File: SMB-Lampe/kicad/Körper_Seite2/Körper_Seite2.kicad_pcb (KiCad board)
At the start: 2 copper layers, 121.9 x 96.3 mm, 32 parts, among them J1 Conn_01x01_Pin, J2 Conn_01x01_Pin, J3 Conn_01x01_Pin

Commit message: Alle Platinen sind fertig zur Fertigung
Aus diesem Stand folgt das erste fertig leuchtende Pferd
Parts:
- C1, C2, C3, C4, C5, C6, C7, C8, C9: footprint Capacitor_SMD:C_0201_0603Metric -> Capacitor_SMD:C_0603_1608Metric_Pad1.08x0.95mm_HandSolder
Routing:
- net GND: track 351.6 -> 358.0 mm
- net Net-(D8-DOUT): track 34.9 -> 37.5 mm
- net +5V: track 207.2 -> 209.1 mm
- net Net-(D7-DOUT): track 82.5 -> 80.9 mm
- net /Data_OUT_Hinterbein_vorne_Seite1: track 71.5 -> 72.8 mm
- net (no net): track 3.40 -> 2.50 mm
- net Net-(D1-DOUT): track 45.8 -> 46.5 mm
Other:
- board size 121.9 x 96.3 mm -> 281.3 x 135.5 mm

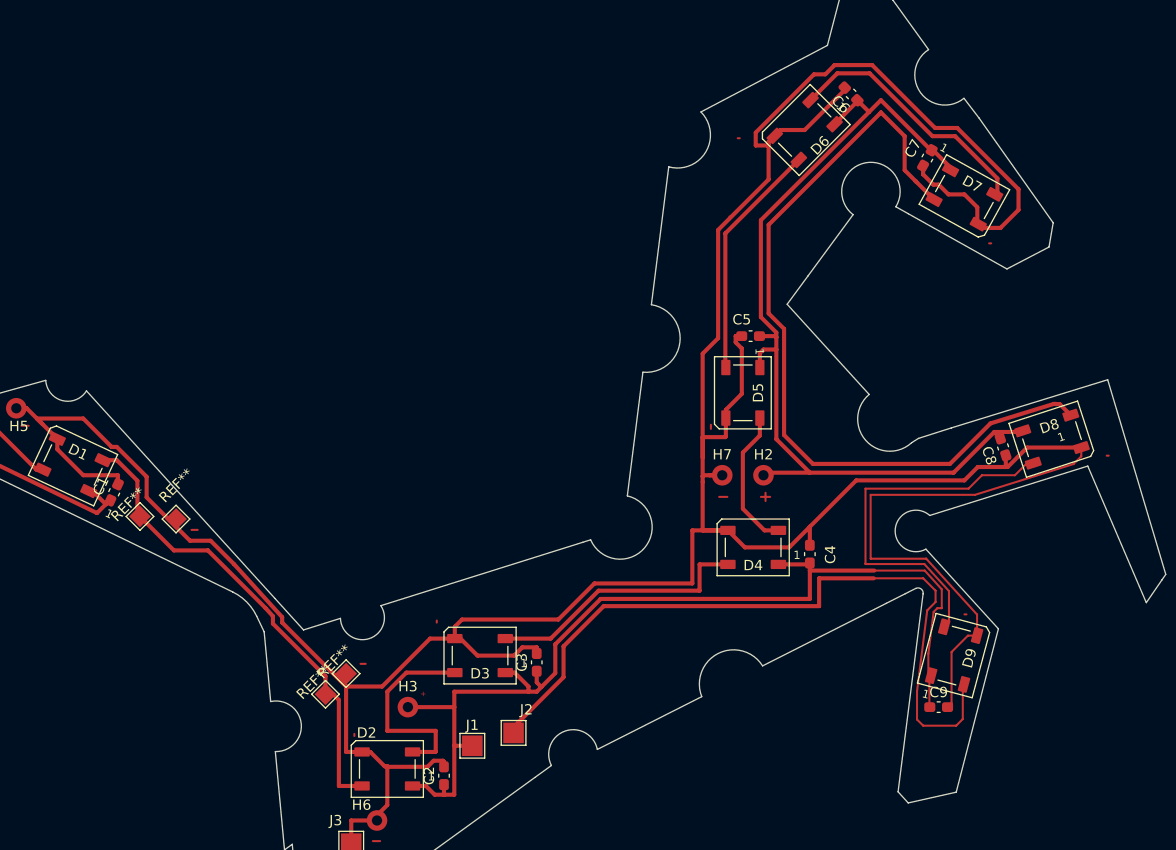
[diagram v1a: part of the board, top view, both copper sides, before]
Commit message: Nachträgliche Änderungen für die Fertigung und Präsentation
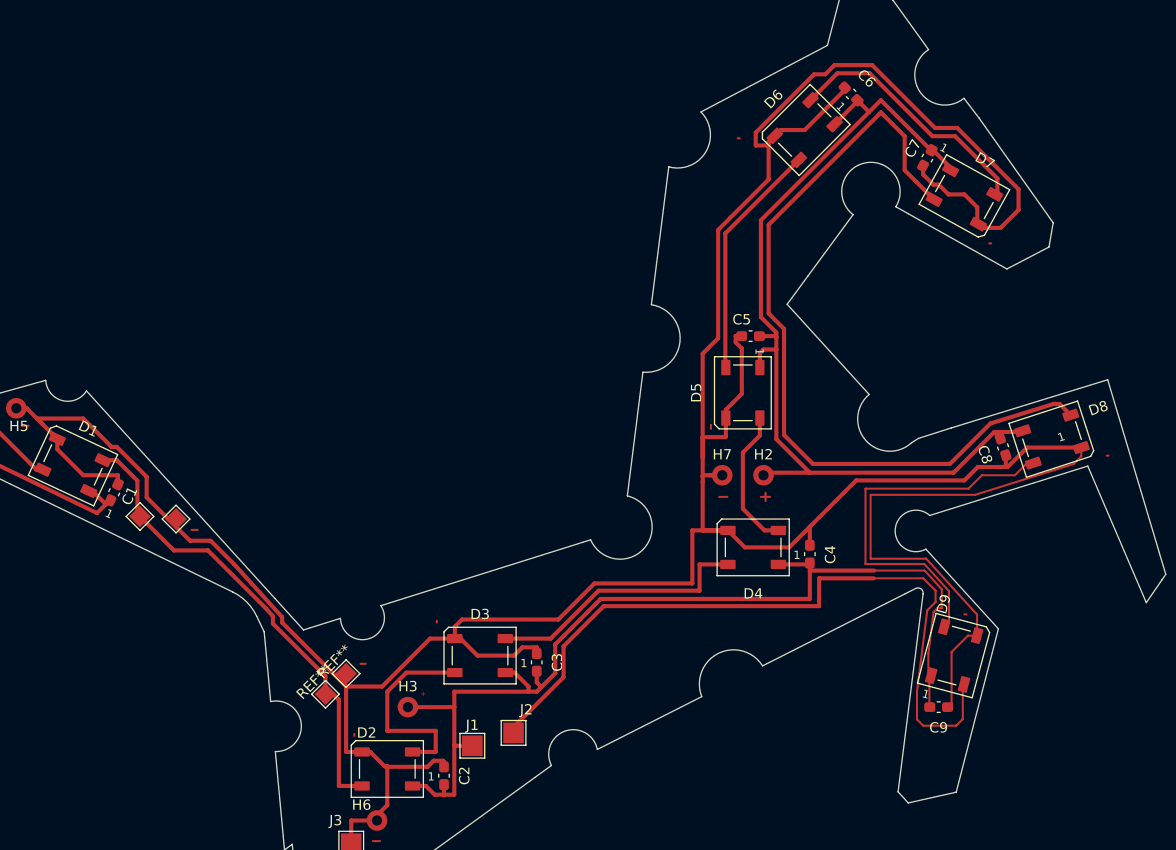
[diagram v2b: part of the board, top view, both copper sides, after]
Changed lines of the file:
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@@
 		(tags "LED RGB NeoPixel PLCC-4 5050")
 		(property "Reference" "D6"
-			(at 0 -2.12132 45)
+			(at 0 4.242641 45)
 			(layer "F.SilkS")
 			(effects
@@
 		(tags "capacitor handsolder")
 		(property "Reference" "C2"
-			(at 0 -1.43 90)
+			(at 0 2 90)
 			(layer "F.SilkS")
 			(effects
@@
 		(tags "LED RGB NeoPixel PLCC-4 5050")
 		(property "Reference" "D9"
-			(at 0.146747 1.513594 75)
+			(at 4.57081 -2.260021 75)
 			(layer "F.SilkS")
 			(effects
@@
 		(tags "capacitor handsolder")
 		(property "Reference" "C6"
-			(at 0 -1.43 135)
+			(at 0 2.12132 135)
 			(layer "F.SilkS")
 			(effects
@@
 		(tags "capacitor handsolder")
 		(property "Reference" "C1"
-			(at 0 -1.43 65)
+			(at 0.321251 1.505265 65)
 			(layer "F.SilkS")
 			(effects
@@
 		(tags "capacitor handsolder")
 		(property "Reference" "C3"
-			(at 0 -1.43 90)
+			(at 0 2 90)
 			(layer "F.SilkS")
 			(effects
@@
 		(tags "LED RGB NeoPixel PLCC-4 5050")
 		(property "Reference" "D8"
-			(at 0.148507 -1.266075 18)
+			(at 5.206805 -1.462593 18)
 			(layer "F.SilkS")
 			(effects
@@
 		(tags "capacitor handsolder")
 		(property "Reference" "C8"
-			(at 0.391225 1.546591 288)
+			(at 0.172513 1.896112 288)
 			(layer "F.SilkS")
 			(effects
@@
 		(tags "LED RGB NeoPixel PLCC-4 5050")
 		(property "Reference" "D4"
-			(at 0 -1.75 0)
+			(at 0 -4.5 0)
 			(layer "F.SilkS")
 			(effects
@@
 		(tags "LED RGB NeoPixel PLCC-4 5050")
 		(property "Reference" "D3"
-			(at 0 -1.75 0)
+			(at 0 4 0)
 			(layer "F.SilkS")
 			(effects
@@
 			(at 2.298097 -2.298097 45)
 			(layer "F.SilkS")
+			(hide yes)
 			(effects
 				(font
@@
 		(tags "LED RGB NeoPixel PLCC-4 5050")
 		(property "Reference" "D5"
-			(at 0 -1.5 90)
+			(at 0 4.5 90)
 			(layer "F.SilkS")
 			(effects
@@
 		(tags "LED RGB NeoPixel PLCC-4 5050")
 		(property "Reference" "D1"
-			(at 0.075119 1.344194 155)
+			(at 0.119702 3.806005 155)
 			(layer "F.SilkS")
 			(effects
@@
 			(at 0 -1.648 45)
 			(layer "F.SilkS")
+			(hide yes)
 			(effects
 				(font
@@
 		(tags "capacitor handsolder")
 		(property "Reference" "C9"
-			(at 0 -1.43 0)
+			(at 0 2 0)
 			(layer "F.SilkS")
 			(effects
@@
 		(tags "LED RGB NeoPixel PLCC-4 5050")
 		(property "Reference" "D7"
-			(at 0.049953 -1.456882 151)
+			(at 0.052406 -4.030788 151)
 			(layer "F.SilkS")
 			(effects
